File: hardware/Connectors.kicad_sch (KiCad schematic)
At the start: 18 parts, among them J1 USB_C_Receptacle_USB2.0, J14 Conn_01x05, J2 M80-5012622, J3 M300-MV31045M1, J4 Harw_Conn_1x2, J5 Harw_Conn_1x2, J6 Harw_Conn_1x4

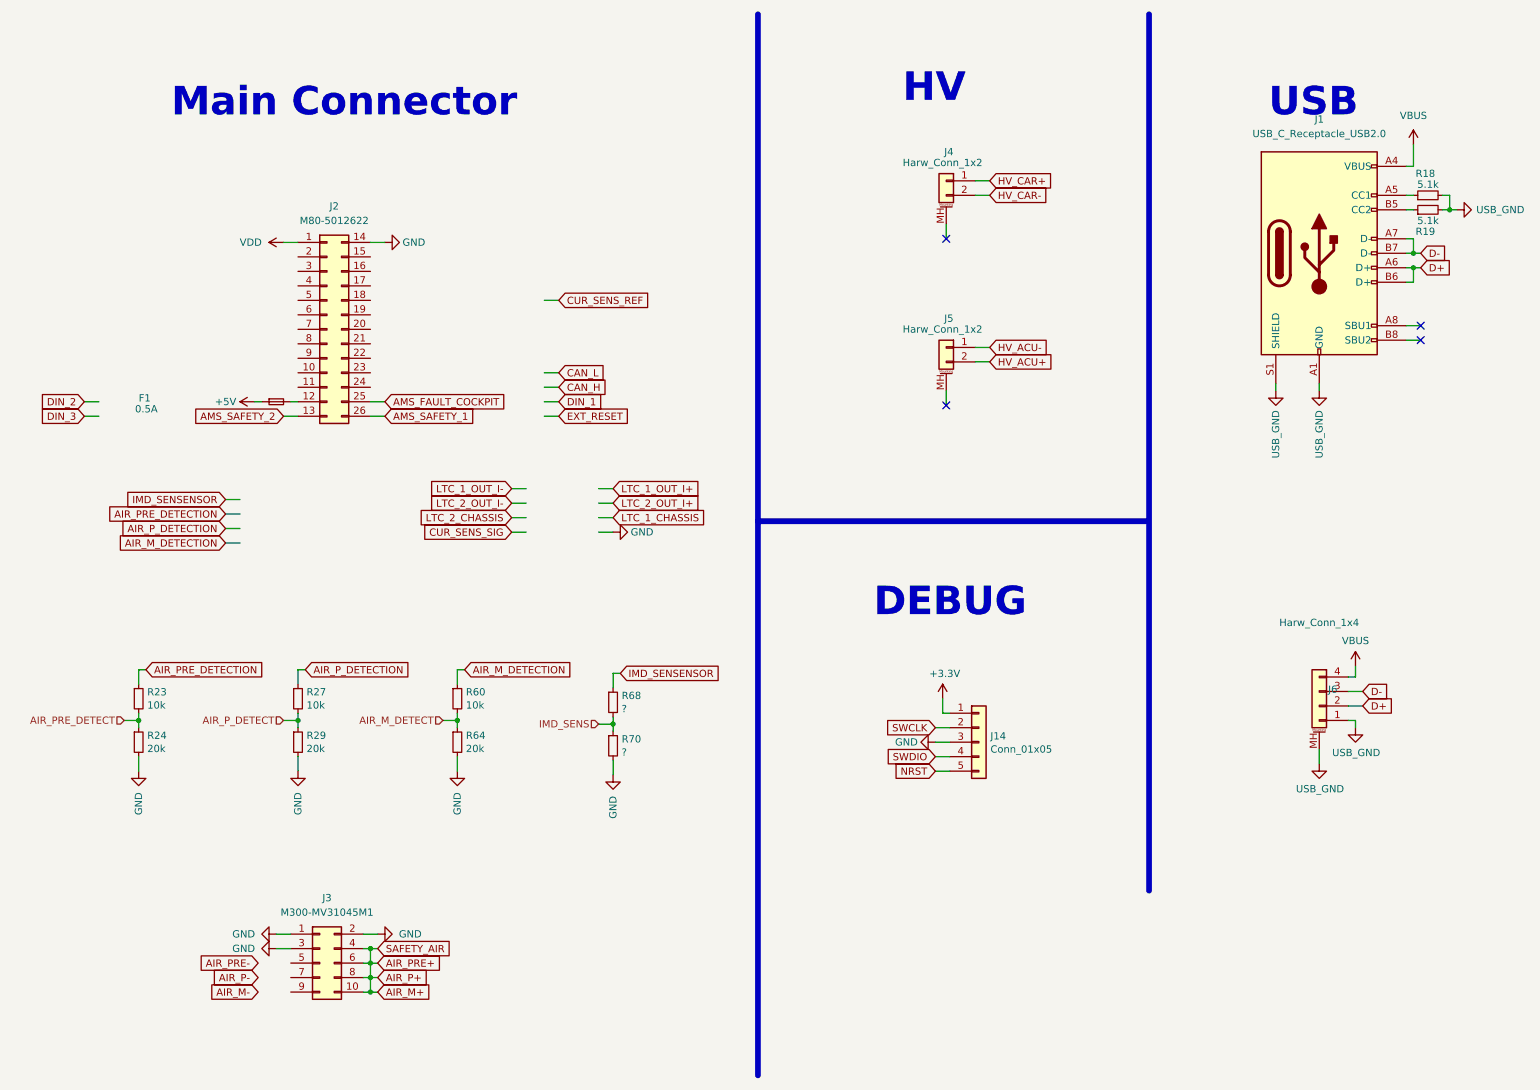
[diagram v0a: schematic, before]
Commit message: changed few connectors, finished board HV section and other minor changes
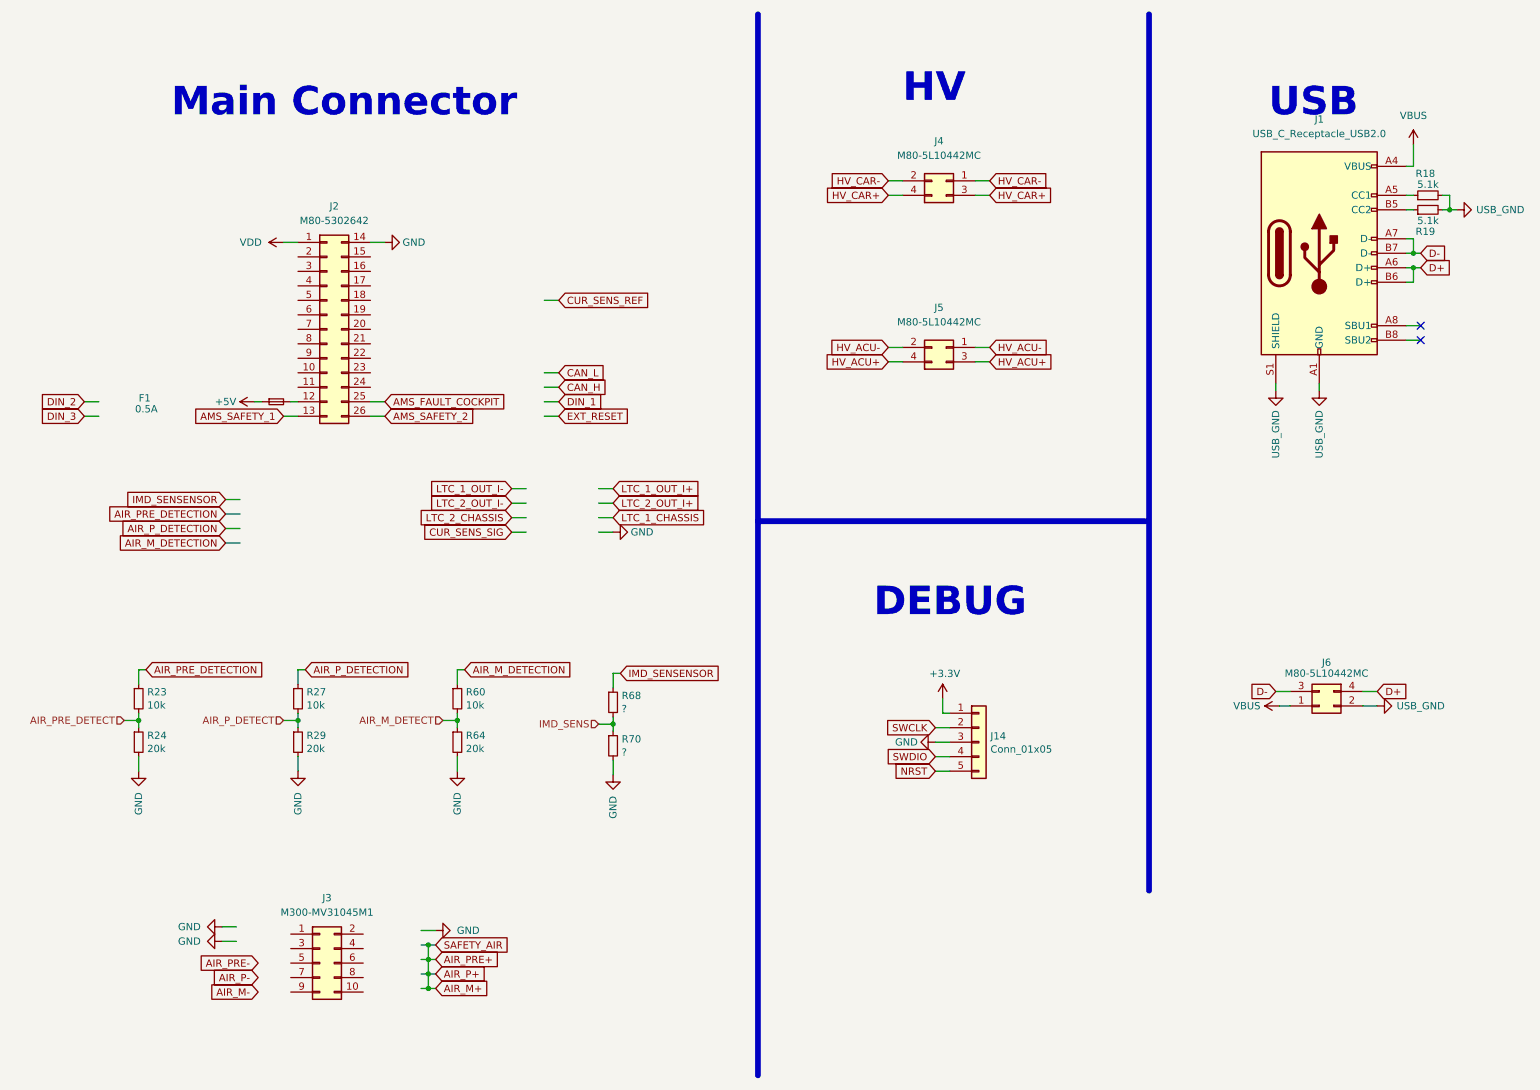
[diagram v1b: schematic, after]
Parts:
- removed J2: M80-5012622, M80-50126YY, symbol M80-5012622:M80-5012622
- removed J4, J5: Harw_Conn_1x2, M808420245, symbol Harwin 2 pin 90 deg:Harw_Conn_1x2
- removed J6: Harw_Conn_1x4, M80-8420445, symbol Harwin 4 pin 90 deg:Harw_Conn_1x4
- added J2: M80-5302642, M80-53026YY, symbol M80-5302642:M80-5302642
- added J4, J5, J6: M80-5L10442MC, M80-5L104YYMC, symbol M80-5L10442MC:M80-5L10442MC
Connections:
- net AIR_M+: no longer J3.10, J3.4, J3.6, J3.8
- net AMS_FAULT_COCKPIT: now also J2.25
- net AMS_SAFETY_1: now also J2.13
- net AMS_SAFETY_2: now also J2.26
- net D+: now also J6.4
- net D-: now also J6.3
- net GND: now also J2.14; no longer J3.1, J3.2, J3.3
- net HV_ACU+: now also J5.3, J5.4
- net HV_ACU-: now also J5.1, J5.2
- net HV_CAR+: now also J4.3, J4.4
- net HV_CAR-: now also J4.1, J4.2
- net USB_GND: now also J6.2
- net VBUS: now also J6.1
- net VDD: now also J2.1
- net at F1.2: now also J2.12
- no-connect marks 4 -> 2
